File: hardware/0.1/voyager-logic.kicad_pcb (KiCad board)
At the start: 6 copper layers, 50 x 50 mm, 156 parts, among them J201 USB_C_Receptacle, J401 UART, J402 JTAG, J501 Probe, SW401 KMR2, U201 USBLC6-2SC6, U202 HD3SS3220, U203 TPD4EUSB30, U204 TPD4EUSB30, U301 CYUSB3014-BZXx, U302 M24M02, U501 SN74LVC245A, U502 SN74LVC245A, U701 TLV62569DRLR, U703 TLV62569DRLR, U704 TLV62569DRLR, Y301 19.2MHz

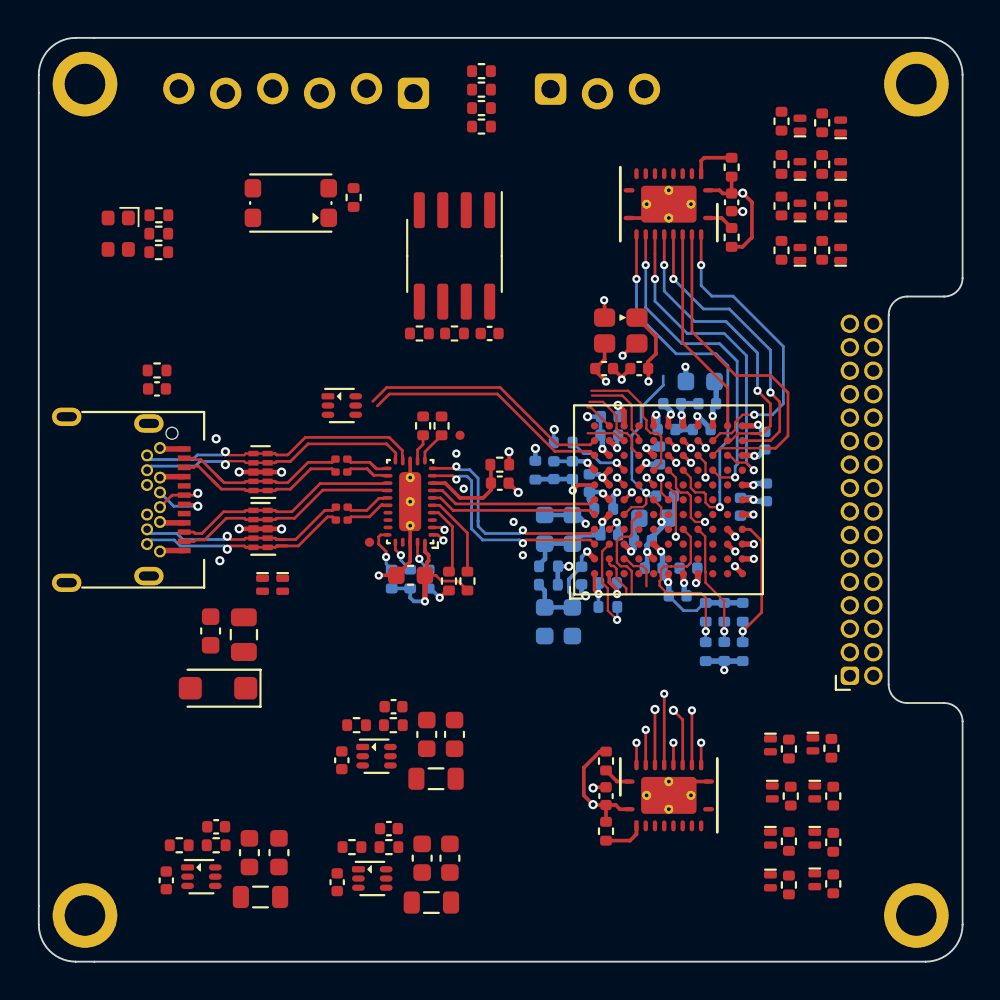
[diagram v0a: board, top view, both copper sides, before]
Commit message: wip, switchers todo
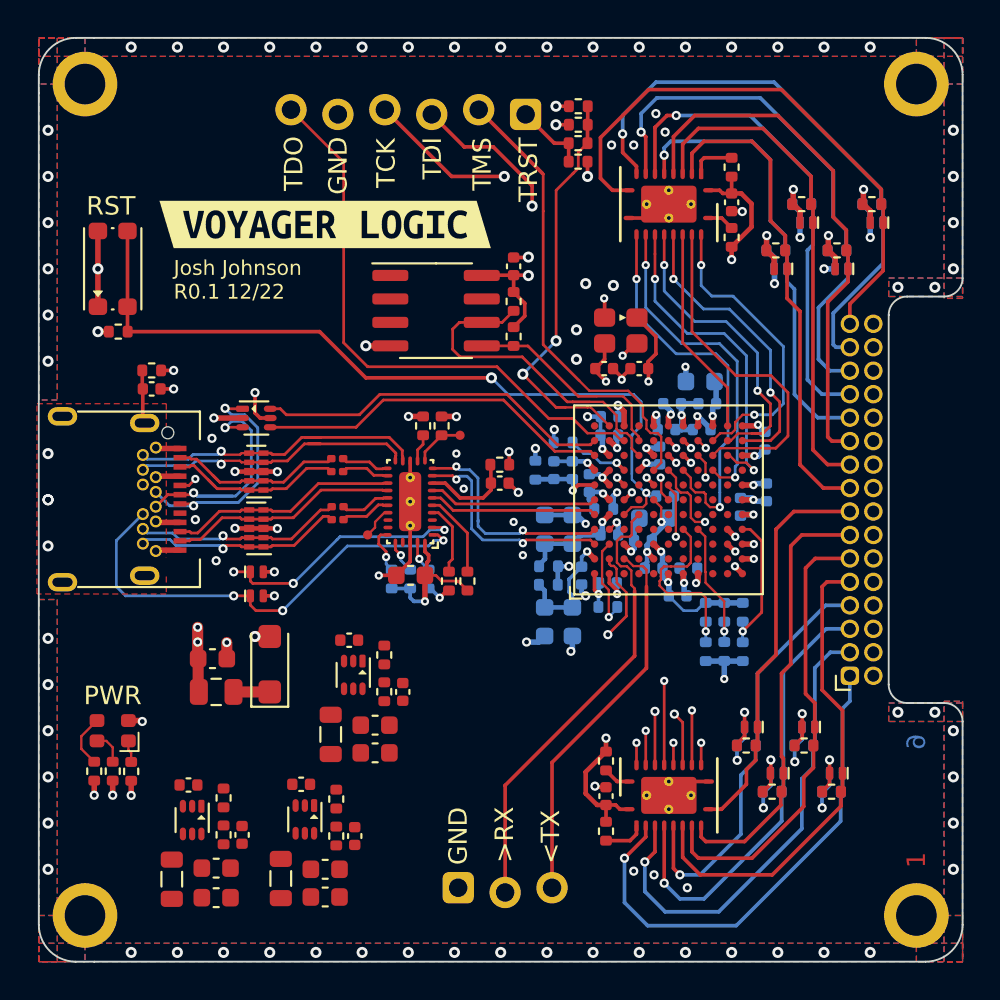
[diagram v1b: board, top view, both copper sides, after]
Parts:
- added G***: LOGO, LOGO, B.Cu at (120.4, 81.9)
- added kibuzzard-63948718: G***, kibuzzard-63948718, F.Cu at (123.0, 79.1)
- D502, D504, D505, D508, D509, D512, D513, D516, R504, R506, R507, R510, R512, R515, R517, R520: moved to B.Cu
- moved J401 43.5 mm to (130.2, 115.1)
- moved R405 30.1 mm to (112.5, 108.7), turned to -90 degrees
- moved R406 29.2 mm to (111.5, 108.7), turned to -90 degrees
- moved R407 28.3 mm to (110.5, 108.7), turned to -90 degrees
- moved D402 26.9 mm to (111.5, 106.5), turned to 180 degrees
- moved R402 14.7 mm to (111.8, 84.9), turned to 0 degrees
- moved SW401 10.3 mm to (111.5, 81.5), turned to 90 degrees
- moved D512 8.30 mm to (149.2, 106.3), turned to 180 degrees
- moved L702 8.25 mm to (120.6, 114.5), turned to -90 degrees
- moved R515 7.66 mm to (148.9, 107.3), turned to 180 degrees
- moved R408 7.17 mm to (136.7, 75.7)
- moved C721 7.07 mm to (123.0, 115.5), turned to 0 degrees
- moved R506 7.04 mm to (145.8, 107.3), turned to 180 degrees
- moved D504 6.96 mm to (146.1, 106.3), turned to 180 degrees
- moved D516 6.84 mm to (150.7, 108.8), turned to 180 degrees
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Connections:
- net Net-(C208-Pad1) renamed /USB C Connector/SHIELD
- J401 pad 1: /Debug/UART_TX -> GND
- J401 pad 3: GND -> /Debug/UART_TX
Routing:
- net GND: track 64.9 -> 117.2 mm, vias 41 -> 149
- net /Debug/FX3_NRST: track 10.1 -> 42.9 mm, vias 1 -> 2
- net /Logic Front End/CHANNEL_14: track 0.00 -> 31.1 mm, vias 0 -> 1
- net /Logic Front End/CHANNEL_15: track 0.00 -> 30.6 mm
- net /Debug/JTAG_TDO: track 2.15 -> 31.2 mm
- net /Logic Front End/CHANNEL_13: track 0.00 -> 28.9 mm, vias 0 -> 1
- net /Logic Front End/CHANNEL_10: track 0.00 -> 28.8 mm
- net /Logic Front End/CHANNEL_0: track 0.00 -> 27.4 mm, vias 0 -> 1
- net /Logic Front End/CHANNEL_9: track 0.00 -> 27.1 mm
- net /Logic Front End/CHANNEL_8: track 0.00 -> 26.5 mm
- net /Logic Front End/CHANNEL_12: track 0.00 -> 26.4 mm, vias 0 -> 1
- net /Logic Front End/CHANNEL_4: track 0.00 -> 26.2 mm
- net /Logic Front End/CHANNEL_1: track 0.00 -> 25.8 mm, vias 0 -> 1
- net +5V: track 9.86 -> 35.4 mm, vias 2 -> 3
- net VBUS: track 2.66 -> 27.8 mm, vias 0 -> 3
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- added copper zone on F.Cu, net /USB C Connector/SHIELD
- added copper zone on B.Cu, net GND
- added copper zone on F.Cu, net GND
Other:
- board text added: "1"
- board text added: "2"
- board text added: "3"
- board text added: "4"
- board text added: "5"
- board text added: "6"
- board text added: "<TX"
- board text added: ">RX"
- board text added: "Born too late to explore the earth Born too soon to explore the galaxy Born just in time to view ones and zeros"
- board text added: "GND"
- board text added: "Josh Johnson R0.1 12/22"
- board text added: "PWR"
- board text added: "RST"
- board text added: "TCK"
- board text added: "TDI"
- board text added: "TDO"
- board text added: "TMS"
- board text added: "TRST"
